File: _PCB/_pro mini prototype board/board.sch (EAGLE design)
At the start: 37 parts, among them T1_5MM 5mm, T2_5MM 5mm, T3_5MM 5mm

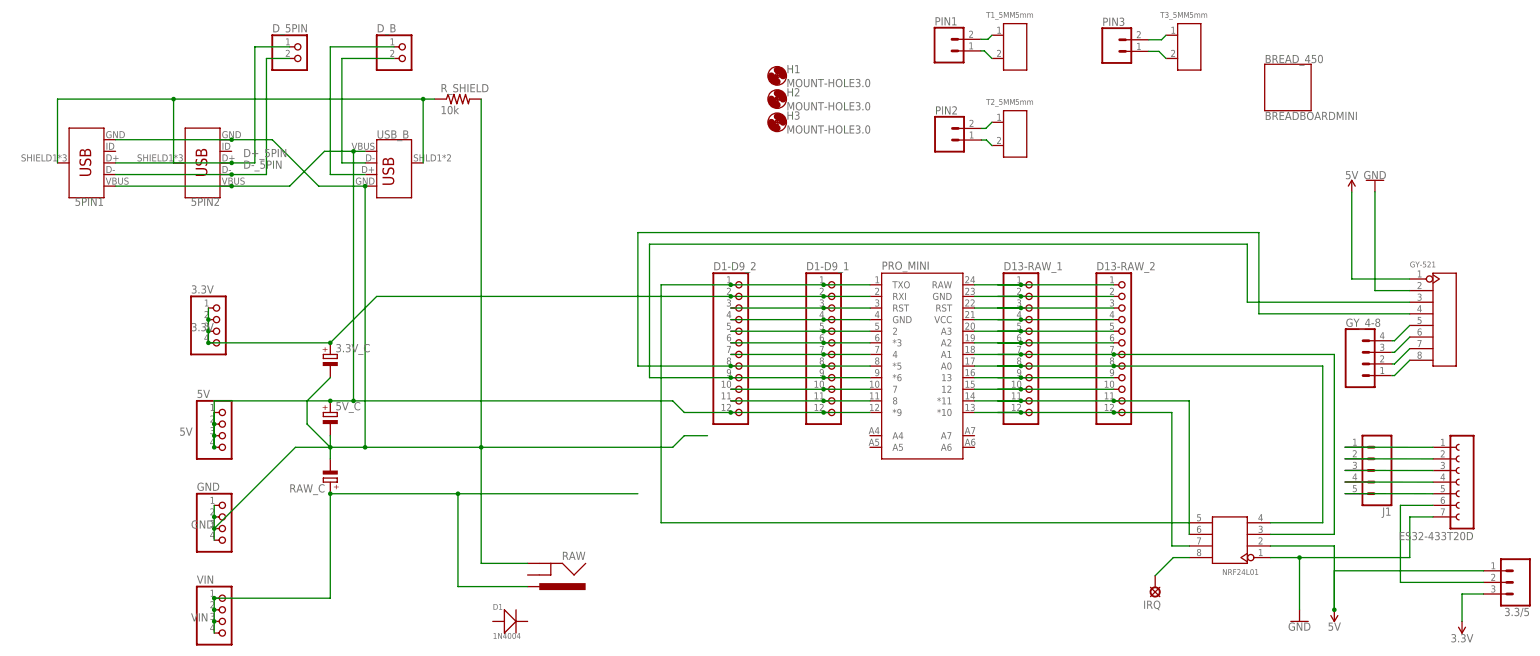
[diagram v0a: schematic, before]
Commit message: library update
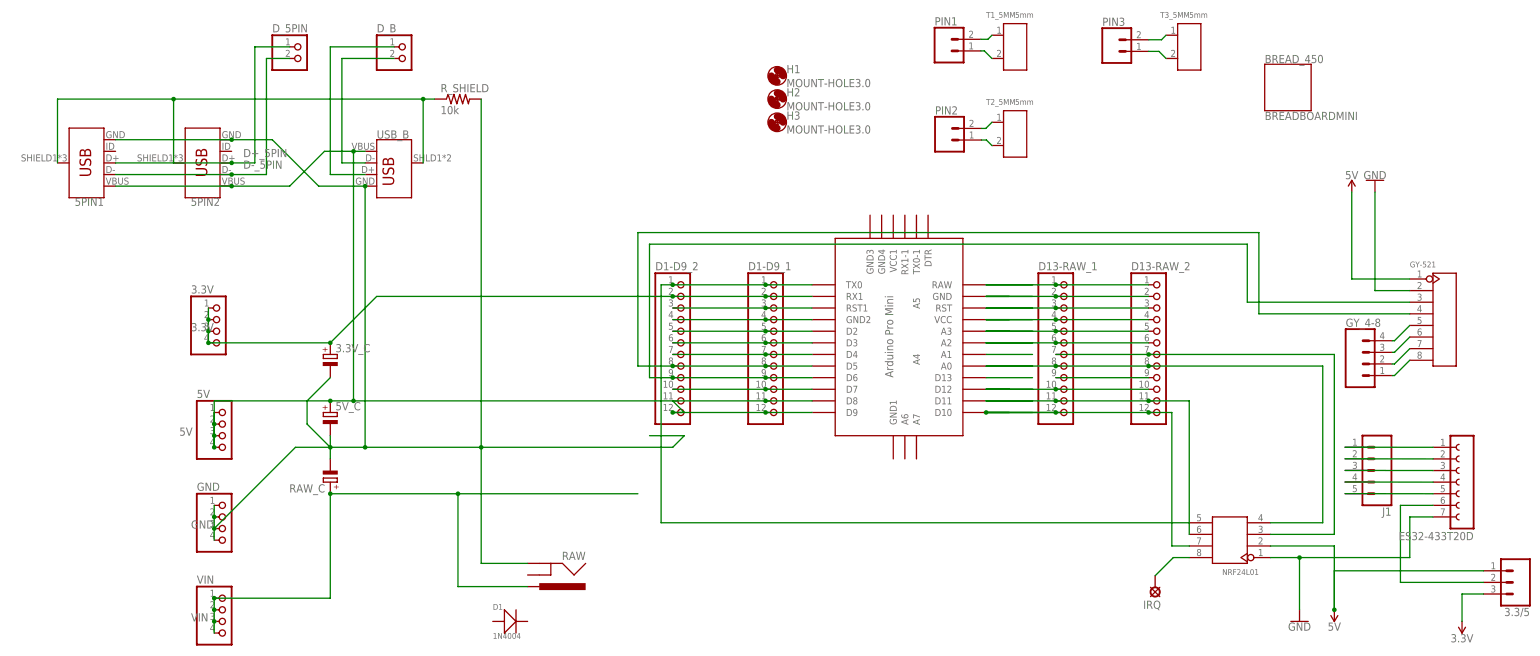
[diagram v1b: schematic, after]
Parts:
- removed PRO_MINI: ARDUINO_PRO_MINI, SparkFun-Boards:ARDUINO_PRO_MINI
- added U$1: ABK-PRO-MINI, Arduino-clone:ABK-PRO-MINI
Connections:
- new net N$28: U$1.A1
- new net N$29: U$1.D13
- net 3.3V: now also U$1.RX1; no longer PRO_MINI.RXI
- net 5V: now also U$1.D9; no longer PRO_MINI.*9
- net A5: now also U$1.D6; no longer PRO_MINI.*6
- net A6: now also U$1.D7; no longer PRO_MINI.7
- net A7: now also U$1.D8; no longer PRO_MINI.8
- net CE_NRF: no longer PRO_MINI.A1
- net CSN_NRF: now also U$1.A0; no longer PRO_MINI.A0
- net MISO_NRF: now also U$1.D10; no longer PRO_MINI.*10
- net MOSI_NRF: now also U$1.D11; no longer PRO_MINI.*11
- net N$16: now also U$1.RAW; no longer PRO_MINI.RAW
- net N$17: now also U$1.GND; no longer PRO_MINI.GND@2
- net N$18: now also U$1.RST; no longer PRO_MINI.RST@2
- net N$19: now also U$1.VCC; no longer PRO_MINI.VCC
- net N$20: now also U$1.A3; no longer PRO_MINI.A3
- net N$21: now also U$1.A2; no longer PRO_MINI.A2
- net N$24: no longer PRO_MINI.13
- net N$25: now also U$1.D12; no longer PRO_MINI.12
- net N$3: now also U$1.RST1; no longer PRO_MINI.RST
- net N$4: now also U$1.GND2; no longer PRO_MINI.GND
- net N$5: now also U$1.D2; no longer PRO_MINI.2
- net N$6: now also U$1.D3; no longer PRO_MINI.*3
- net N$7: now also U$1.D4; no longer PRO_MINI.4
- net SCK_NRF: now also U$1.TX0; no longer PRO_MINI.TXO
- net SDA_GY521: now also U$1.D5; no longer PRO_MINI.*5
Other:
- moved on the sheet: D1-D9_1, D1-D9_2, D13-RAW_1, D13-RAW_2
